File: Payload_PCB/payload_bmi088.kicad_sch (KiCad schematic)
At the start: 3 parts, among them U8 BMI088

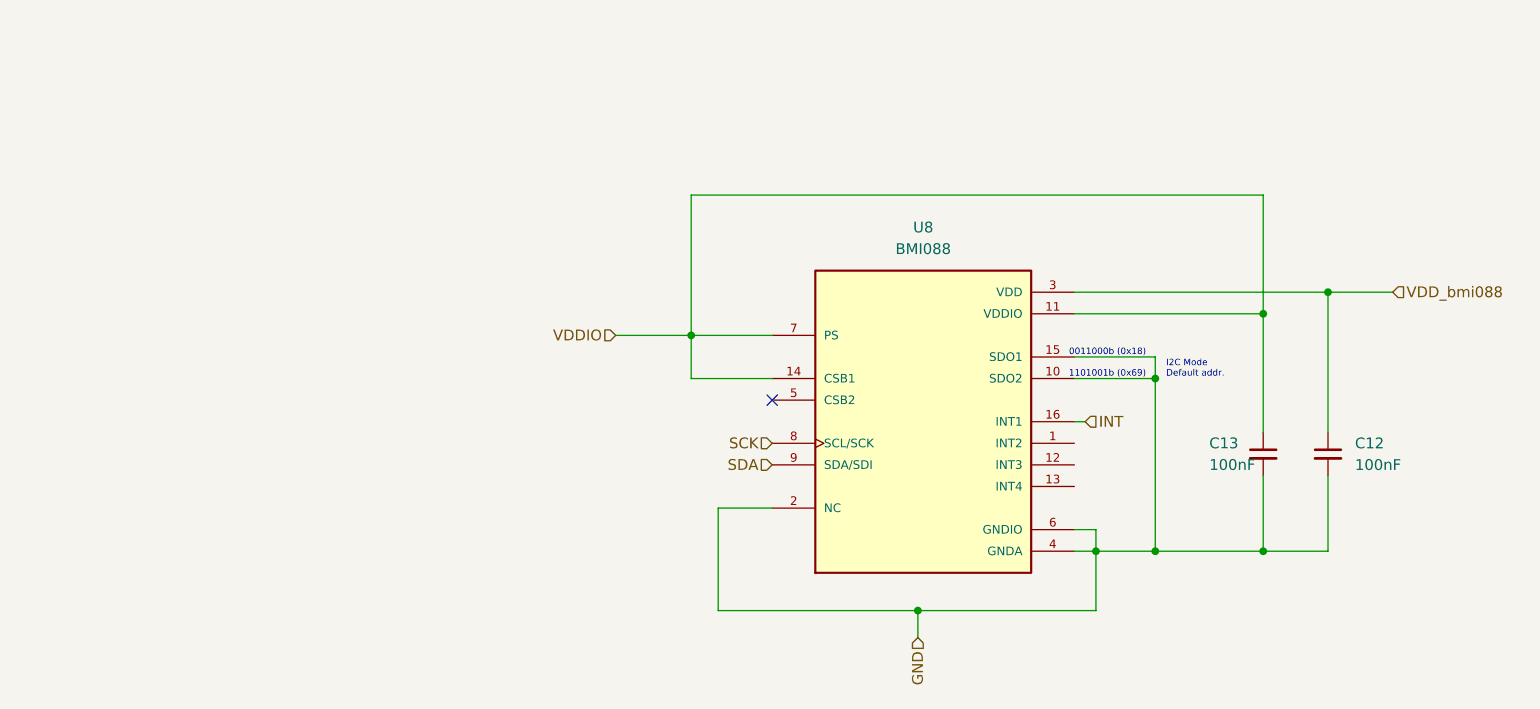
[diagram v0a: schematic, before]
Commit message: Adjust page size
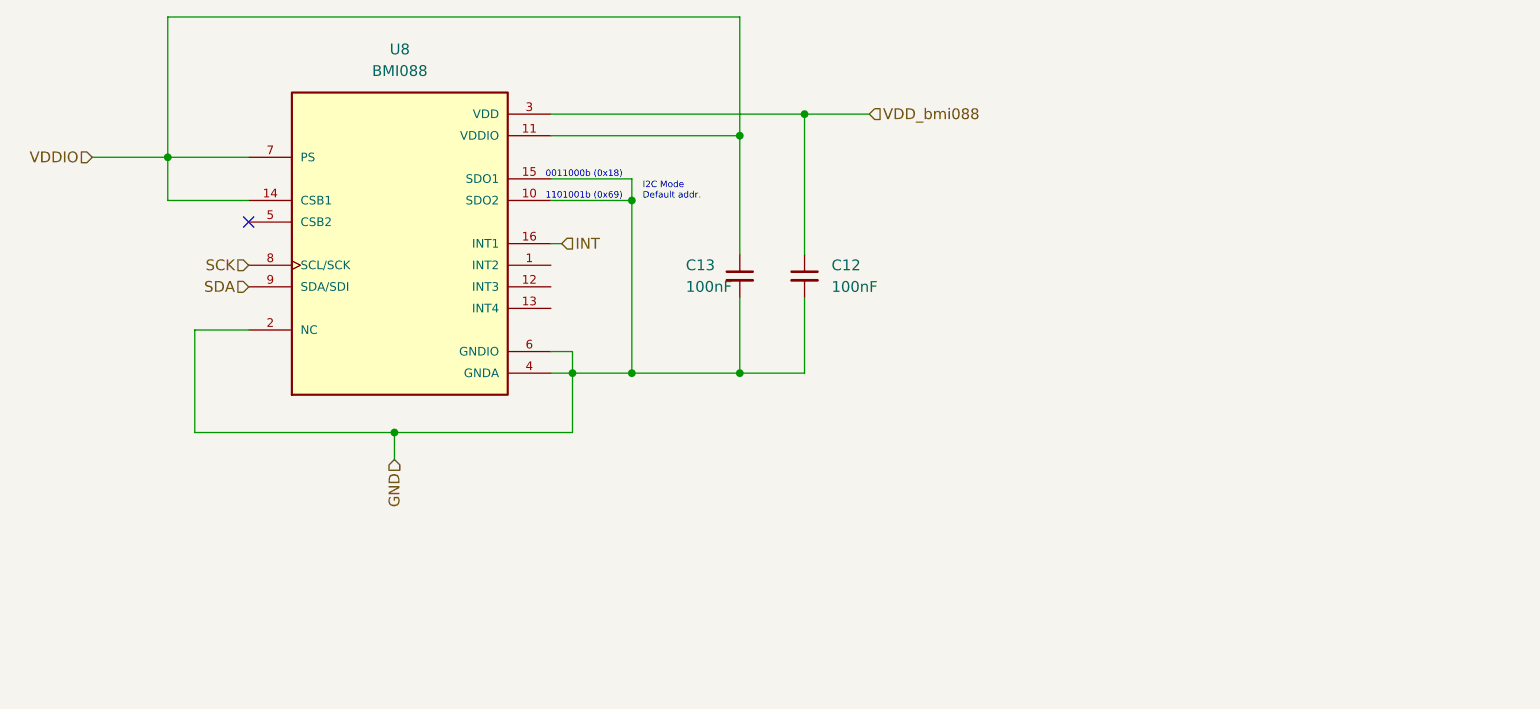
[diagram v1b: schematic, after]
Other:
- moved on the sheet: C12, C13, U8

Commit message: some new parts
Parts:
- U8: footprint BMI088:PQFN50P450X300X100-16N -> footprints:PQFN50P450X300X100-16N
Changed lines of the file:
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@@
       (effects (font (size 1.27 1.27)))
     )
-    (property "Footprint" "BMI088:PQFN50P450X300X100-16N" (at 90.17 65.405 0)
+    (property "Footprint" "footprints:PQFN50P450X300X100-16N" (at 90.17 65.405 0)
       (effects (font (size 1.27 1.27)) (justify bottom) hide)
     )
